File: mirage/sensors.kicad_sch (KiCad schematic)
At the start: 2 parts, among them U2 MS560702BA03-50, U3 ADXL375BCCZ-RL7

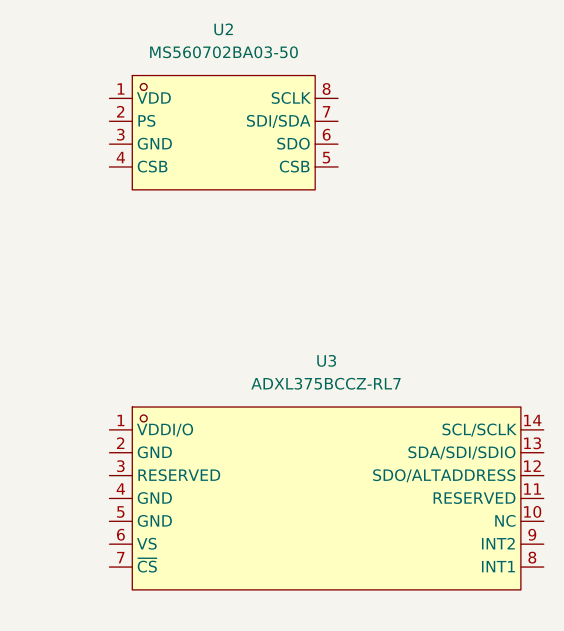
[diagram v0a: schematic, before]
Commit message: feat: initialize structure
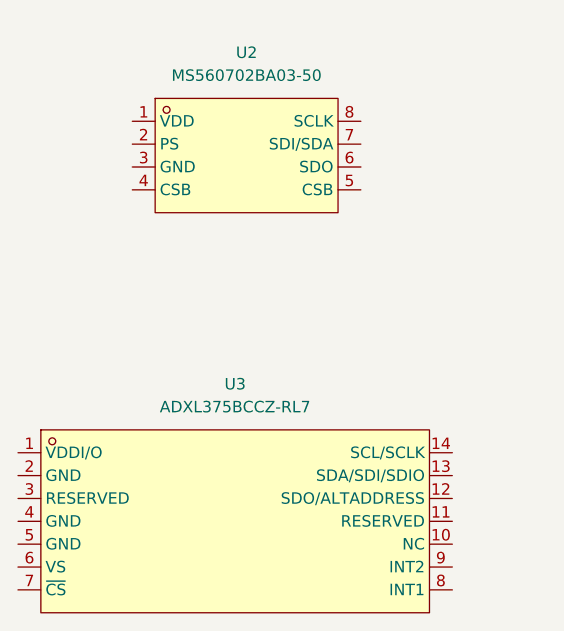
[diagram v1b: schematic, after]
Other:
- moved on the sheet: U2, U3
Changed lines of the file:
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@@
 	(symbol
 		(lib_id "EasyEDA:MS560702BA03-50")
-		(at 67.31 38.1 0)
+		(at 69.85 40.64 0)
 		(unit 1)
 		(exclude_from_sim no)
@@
 		(fields_autoplaced yes)
 		(property "Reference" "U2"
-			(at 67.31 26.67 0)
+			(at 69.85 29.21 0)
 			(effects
 				(font
@@
 		)
 		(property "Value" "MS560702BA03-50"
-			(at 67.31 29.21 0)
+			(at 69.85 31.75 0)
 			(effects
 				(font
@@
 		)
 		(property "Footprint" "EasyEDA:SENSOR-SMD_MS560702BA03-50"
-			(at 67.31 49.53 0)
+			(at 69.85 52.07 0)
 			(effects
 				(font
@@
 		)
 		(property "Datasheet" "https://lcsc.com/product-detail/Pre-ordered-Products_TE-Connectivity_MS560702BA03-50_TE-Connectivity-MS560702BA03-50_C97627.html"
-			(at 67.31 52.07 0)
+			(at 69.85 54.61 0)
 			(effects
 				(font
@@
 		)
 		(property "Description" ""
-			(at 67.31 38.1 0)
+			(at 69.85 40.64 0)
 			(effects
 				(font
@@
 		)
 		(property "LCSC Part" "C97627"
-			(at 67.31 54.61 0)
+			(at 69.85 57.15 0)
 			(effects
 				(font
@@
 	(symbol
 		(lib_id "EasyEDA:ADXL375BCCZ-RL7")
-		(at 78.74 78.74 0)
+		(at 68.58 81.28 0)
 		(unit 1)
 		(exclude_from_sim no)
@@
 		(fields_autoplaced yes)
 		(property "Reference" "U3"
-			(at 78.74 63.5 0)
+			(at 68.58 66.04 0)
 			(effects
 				(font
@@
 		)
 		(property "Value" "ADXL375BCCZ-RL7"
-			(at 78.74 66.04 0)
+			(at 68.58 68.58 0)
 			(effects
 				(font
@@
 		)
 		(property "Footprint" "EasyEDA:LGA-14_L5.0-W3.0-P0.80-BL"
-			(at 78.74 93.98 0)
+			(at 68.58 96.52 0)
 			(effects
 				(font
@@
 		)
 		(property "Datasheet" "https://lcsc.com/product-detail/New-Arrivals_Analog-Devices-ADI-ADXL375BCCZ-RL7_C481898.html"
-			(at 78.74 96.52 0)
+			(at 68.58 99.06 0)
 			(effects
 				(font
@@
 		)
 		(property "Description" ""
-			(at 78.74 78.74 0)
+			(at 68.58 81.28 0)
 			(effects
 				(font
@@
 		)
 		(property "LCSC Part" "C481898"
-			(at 78.74 99.06 0)
+			(at 68.58 101.6 0)
 			(effects
 				(font
